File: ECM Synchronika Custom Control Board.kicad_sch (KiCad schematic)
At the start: 0 parts

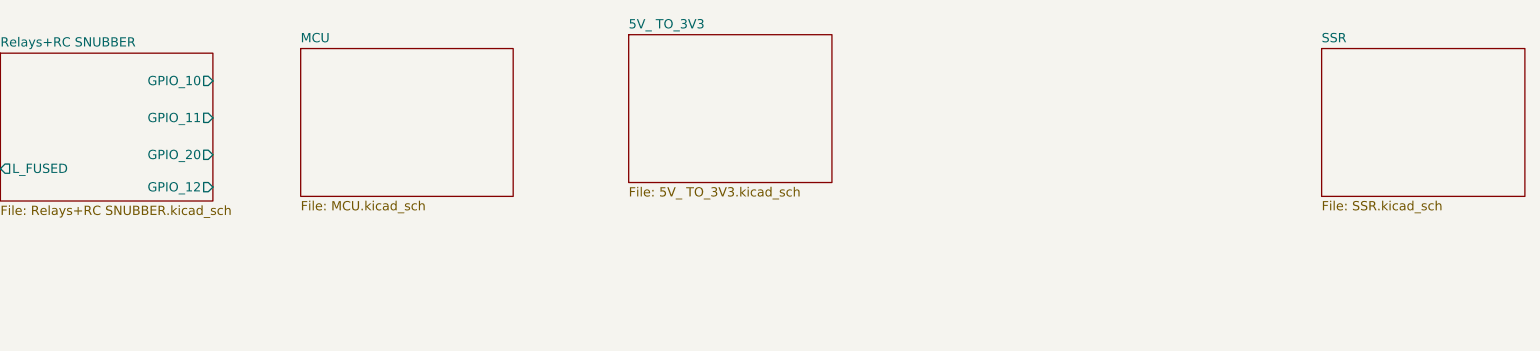
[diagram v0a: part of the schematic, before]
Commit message: SCHEMATIC CONTINUATION
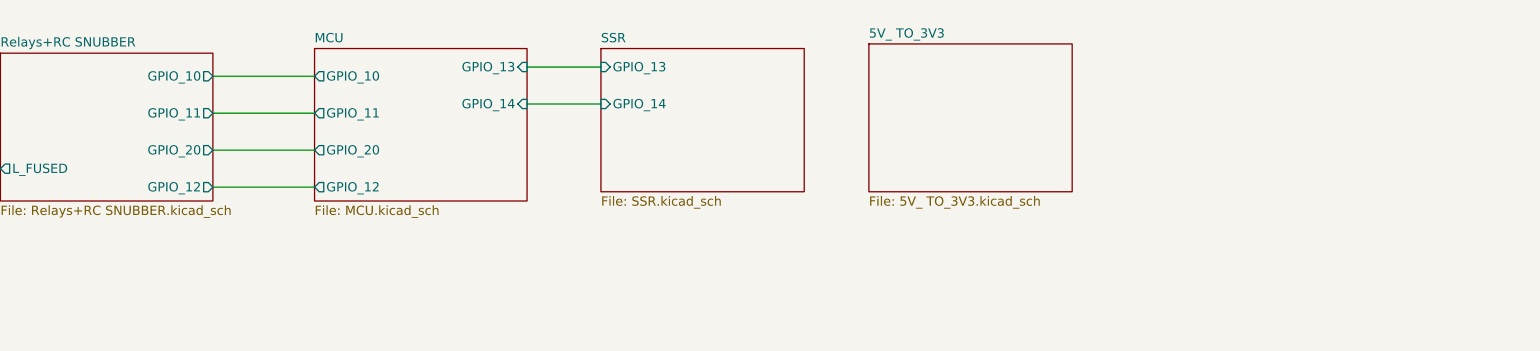
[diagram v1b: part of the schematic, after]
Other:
- sheet MCU ports: added GPIO_10, GPIO_11, GPIO_12, GPIO_13, GPIO_14, GPIO_20; removed none
- sheet SSR ports: added GPIO_13, GPIO_14; removed none
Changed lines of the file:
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@@
+	(wire
+		(pts
+			(xy 82.55 25.4) (xy 96.52 25.4)
+		)
+		(stroke
+			(width 0)
+			(type default)
+		)
+	)
+	(wire
+		(pts
+			(xy 82.55 35.56) (xy 96.52 35.56)
+		)
+		(stroke
+			(width 0)
+			(type default)
+		)
+	)
+	(wire
+		(pts
+			(xy 125.73 24.13) (xy 135.89 24.13)
+		)
+		(stroke
+			(width 0)
+			(type default)
+		)
+	)
+	(wire
+		(pts
+			(xy 82.55 30.48) (xy 96.52 30.48)
+		)
+		(stroke
+			(width 0)
+			(type default)
+		)
+	)
+	(wire
+		(pts
+			(xy 82.55 20.32) (xy 96.52 20.32)
+		)
+		(stroke
+			(width 0)
+			(type default)
+		)
+	)
 	(wire
 		(pts
 			(xy 40.64 33.02) (xy 53.34 33.02)
+		)
+		(stroke
+			(width 0)
+			(type default)
+		)
+	)
+	(wire
+		(pts
+			(xy 125.73 19.05) (xy 135.89 19.05)
 		)
 		(stroke
@@
 		)
 		(pin "GPIO_10" output
-			(at 82.55 20.955 0)
+			(at 82.55 20.32 0)
 			(effects
 				(font
@@
 		)
 		(pin "GPIO_11" output
-			(at 82.55 26.035 0)
+			(at 82.55 25.4 0)
 			(effects
 				(font
@@
 		)
 		(pin "GPIO_20" output
-			(at 82.55 31.115 0)
+			(at 82.55 30.48 0)
 			(effects
 				(font
@@
 	)
 	(sheet
-		(at 234.95 16.51)
-		(size 27.94 20.32)
+		(at 135.89 16.51)
+		(size 27.94 19.685)
 		(exclude_from_sim no)
 		(in_bom yes)
@@
 		)
 		(property "Sheetname" "SSR"
-			(at 234.95 15.7984 0)
+			(at 135.89 15.7984 0)
 			(effects
 				(font
@@
 		)
 		(property "Sheetfile" "SSR.kicad_sch"
-			(at 234.95 37.4146 0)
-			(effects
-				(font
-					(size 1.27 1.27)
-				)
-				(justify left top)
+			(at 135.89 36.7796 0)
+			(effects
+				(font
+					(size 1.27 1.27)
+				)
+				(justify left top)
+			)
+		)
+		(pin "GPIO_13" input
+			(at 135.89 19.05 180)
+			(effects
+				(font
+					(size 1.27 1.27)
+				)
+				(justify left)
+			)
+		)
+		(pin "GPIO_14" input
+			(at 135.89 24.13 180)
+			(effects
+				(font
+					(size 1.27 1.27)
+				)
+				(justify left)
 			)
 		)
@@
 	)
 	(sheet
-		(at 139.7 14.605)
+		(at 172.72 15.875)
 		(size 27.94 20.32)
 		(exclude_from_sim no)
@@
 		)
 		(property "Sheetname" "5V_ TO_3V3"
-			(at 139.7 13.8934 0)
+			(at 172.72 15.1634 0)
 			(effects
 				(font
@@
 		)
 		(property "Sheetfile" "5V_ TO_3V3.kicad_sch"
-			(at 139.7 35.5096 0)
+			(at 172.72 36.7796 0)
 			(effects
 				(font
@@
 	)
 	(sheet
-		(at 94.615 16.51)
-		(size 29.21 20.32)
+		(at 96.52 16.51)
+		(size 29.21 20.955)
 		(exclude_from_sim no)
 		(in_bom yes)
@@
 		)
 		(property "Sheetname" "MCU"
-			(at 94.615 15.7984 0)
+			(at 96.52 15.7984 0)
 			(effects
 				(font
@@
 		)
 		(property "Sheetfile" "MCU.kicad_sch"
-			(at 94.615 37.4146 0)
-			(effects
-				(font
-					(size 1.27 1.27)
-				)
-				(justify left top)
-			)
-		)
+			(at 96.52 38.0496 0)
+			(effects
+				(font
+					(size 1.27 1.27)
+				)
+				(justify left top)
+			)
+		)
+		(pin "GPIO_10" output
+			(at 96.52 20.32 180)
+			(effects
+				(font
+					(size 1.27 1.27)
+				)
+				(justify left)
+			)
+		)
+		(pin "GPIO_11" output
+			(at 96.52 25.4 180)
+			(effects
+				(font
+					(size 1.27 1.27)
+				)
+				(justify left)
+			)
+		)
+		(pin "GPIO_12" output
+			(at 96.52 35.56 180)
+			(effects
+				(font
+					(size 1.27 1.27)
+				)
+				(justify left)
+			)
+		)
+		(pin "GPIO_20" output
+			(at 96.52 30.48 180)
+			(effects
+				(font
+					(size 1.27 1.27)
+				)
+				(justify left)
+			)
+		)
+		(pin "GPIO_13" input
+			(at 125.73 19.05 0)
+			(effects
+				(font
+					(size 1.27 1.27)
+				)
+				(justify right)
+			)
+		)
+		(pin "GPIO_14" input
+			(at 125.73 24.13 0)
+			(effects
+				(font
+					(size 1.27 1.27)
+				)
+				(justify right)
+			)
+		)
